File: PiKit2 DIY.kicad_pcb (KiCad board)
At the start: 2 copper layers, 56.9 x 66.3 mm, 38 parts, among them J1 Conn_01x06_Socket, J4 USB_C_Receptacle_USB2.0_16P, Q1 2N3904, Q2 2N3904, Q3 2N3906, Q4 2N3904, SW1 SW_Push, U1 PIC18F2550-ISP, X1 20Mhz

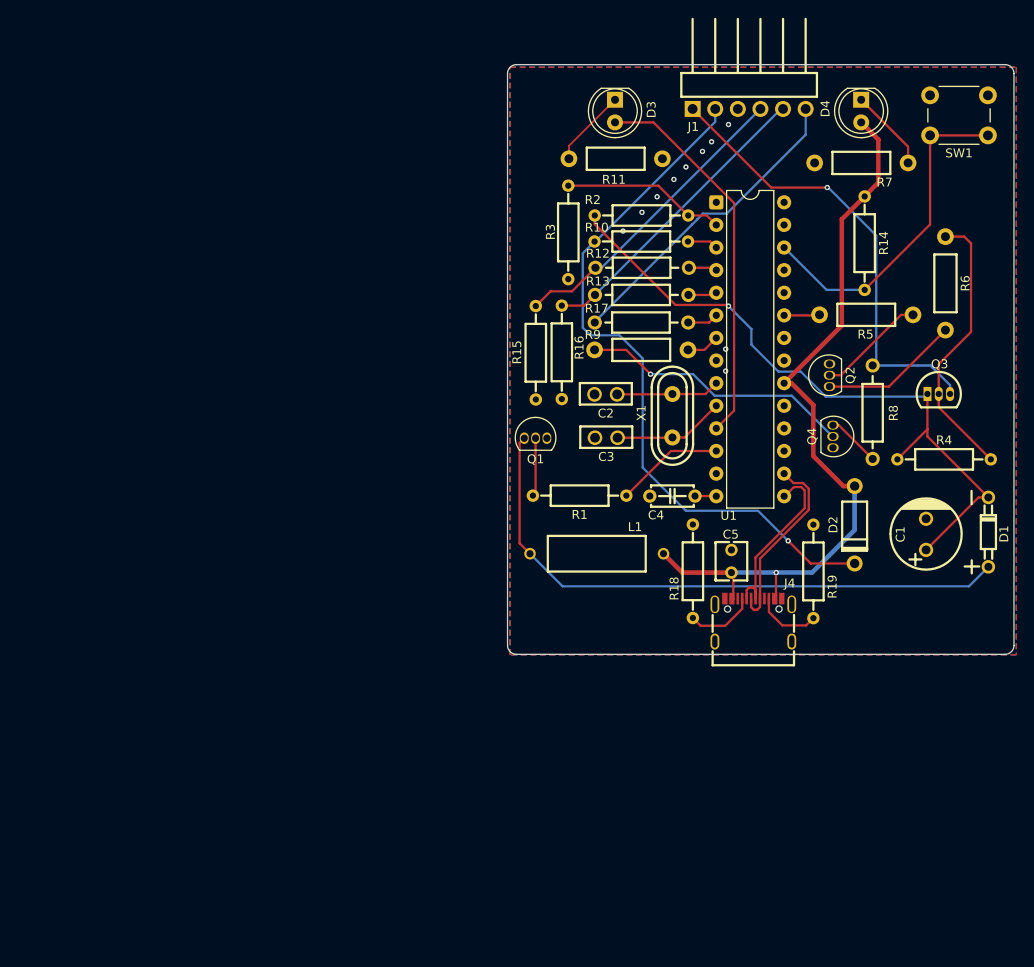
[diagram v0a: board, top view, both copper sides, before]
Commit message: Update to images
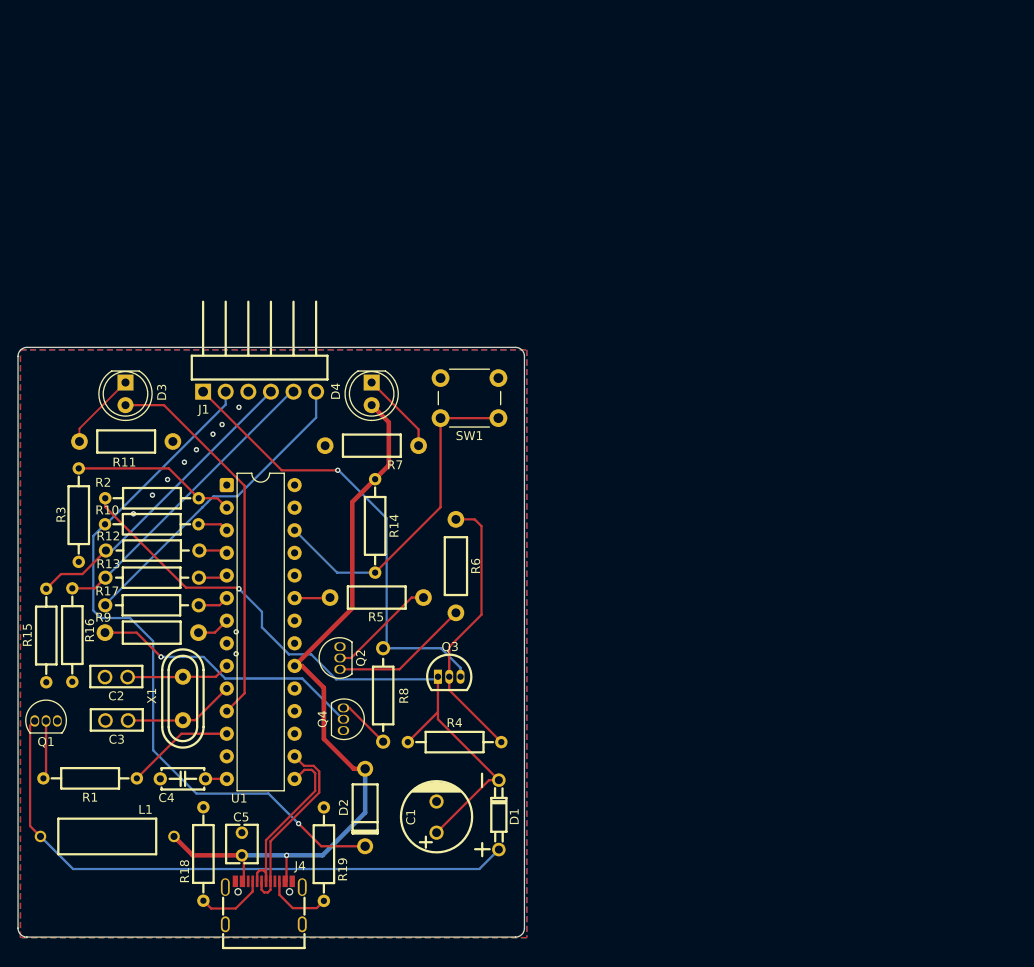
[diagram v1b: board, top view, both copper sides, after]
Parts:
- moved Q4 63.5 mm to (146.4, 100.7)
- moved R7 63.5 mm to (149.6, 70.0)
- moved SW1 63.5 mm to (163.8, 66.9)
- moved C2 63.5 mm to (120.9, 96.0)
- moved D3 63.5 mm to (121.9, 62.9)
- moved R1 63.5 mm to (117.9, 107.3)
- moved R13 63.5 mm to (124.9, 84.8)
- moved R3 63.5 mm to (116.7, 77.8)
- moved R16 63.5 mm to (115.9, 91.2)
- moved C1 63.5 mm to (156.9, 111.7)
- moved C3 63.5 mm to (120.9, 100.8)
- moved C4 63.5 mm to (128.4, 107.4)
- moved C5 63.5 mm to (135.0, 114.7)
- moved D1 63.5 mm to (163.9, 111.4)
- moved D2 63.5 mm to (148.8, 110.6)
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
